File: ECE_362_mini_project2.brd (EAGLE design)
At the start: 71.1 x 35.2 mm, 18 parts

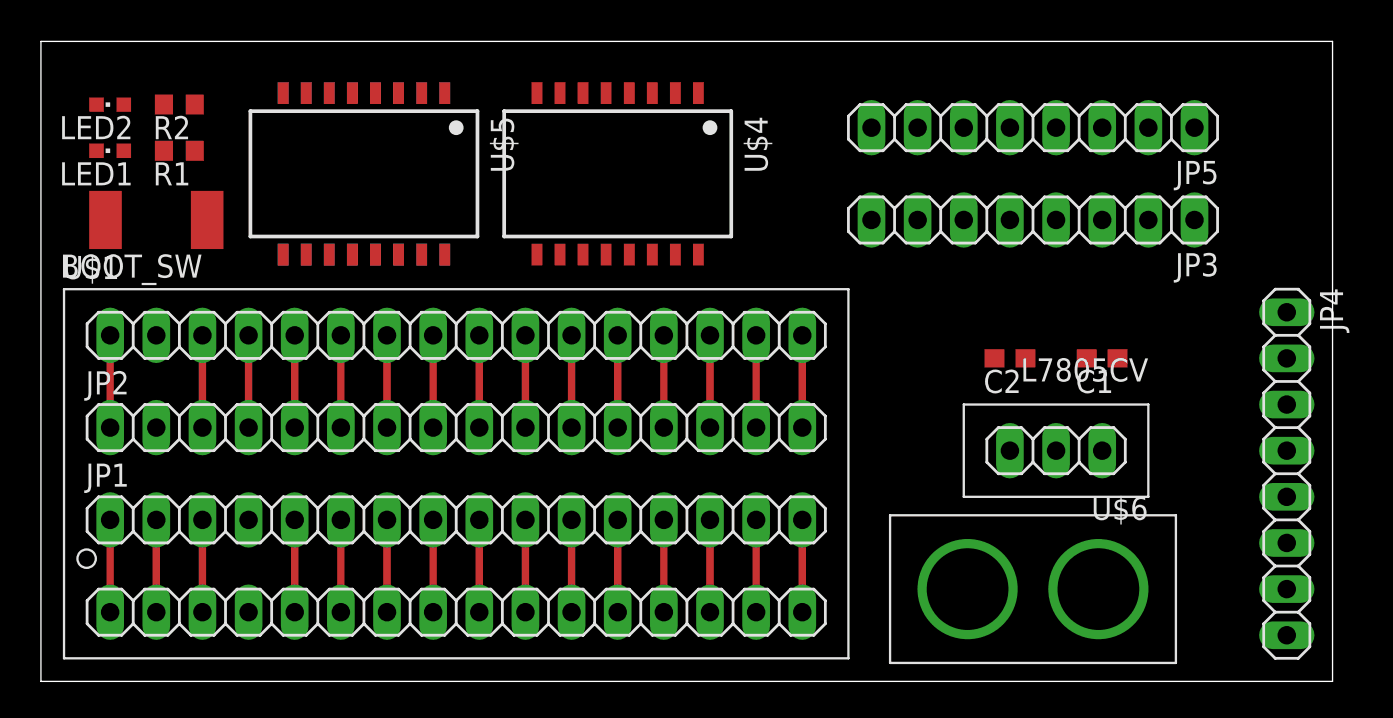
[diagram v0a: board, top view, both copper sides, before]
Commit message: Updated the board
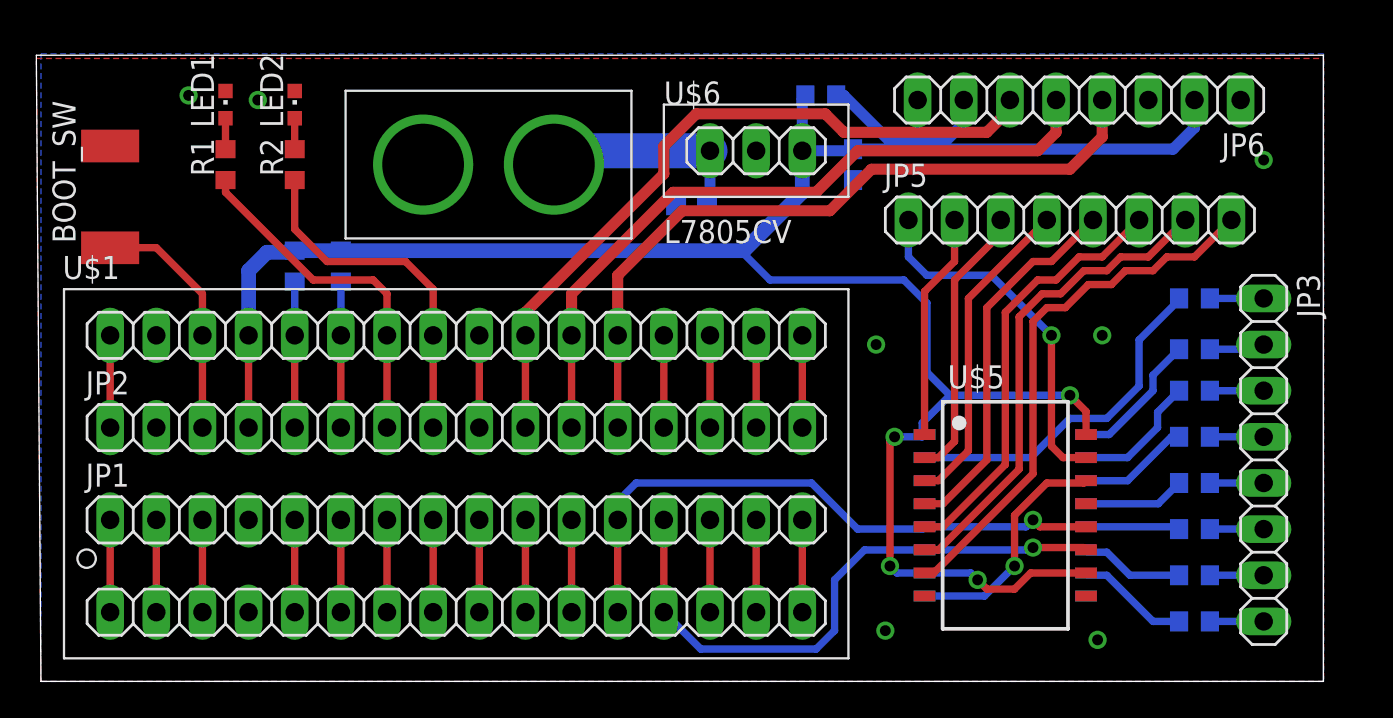
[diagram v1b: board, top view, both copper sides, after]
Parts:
- removed JP4: (no value), pinhead:1X08
- removed U$4: SHIFT_REGISTER, mini_project_parts:N5
- added JP6: (no value), pinhead:1X08
- added R10, R11, R12, R20, R5, R6, R7, R8, R9: 220, resistor:R0603
- added R3, R4: 10k, resistor:R0603
- moved U$2 40.0 mm to (53.1, 9.14), turned to 270 degrees
- moved U$5 40.0 mm to (53.1, 9.14), turned to 270 degrees
- moved U$3 38.0 mm to (24.6, 28.4)
- moved U$6 29.0 mm to (34.3, 26.7), turned to 0 degrees
- moved C1 24.1 mm to (35.8, 26.2), flipped to the bottom
- moved JP3 18.3 mm to (67.3, 12.2), turned to 270 degrees
- moved C2 13.7 mm to (44.7, 28.4), flipped to the bottom, turned to 270 degrees
- moved LED2 10.2 mm to (14.0, 31.8), turned to 0 degrees
- moved R2 7.16 mm to (14.0, 28.4), turned to 90 degrees
- moved LED1 6.84 mm to (10.2, 31.8), turned to 0 degrees
- moved JP5 5.47 mm to (56.6, 25.4), turned to 0 degrees
- moved BOOT_SW 2.84 mm to (3.81, 26.7), turned to 90 degrees
- moved R1 2.65 mm to (10.2, 28.4), turned to 90 degrees
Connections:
- removed net LED2_Q0: JP4.1, U$2.9, U$4.15
- removed net LED2_Q1: JP4.2, U$4.1
- removed net LED2_Q2: JP4.3, U$4.2
- removed net LED2_Q3: JP4.4, U$4.3
- removed net LED2_Q4: JP4.5, U$4.4
- removed net LED2_Q5: JP4.6, U$4.5
- removed net LED2_Q6: JP4.7, U$4.6
- removed net LED2_Q7: JP4.8, U$4.7
- new net A0: R20.1, U$2.15
- new net A1: R6.1, U$2.1
- new net A2: R7.1, U$2.2
- new net A3: R8.1, U$2.3
- new net A4: R9.1, U$2.4
- new net A5: R10.1, U$2.5
- new net A7: R12.1, U$2.7
- new net N$3: R11.1, U$2.6
- new net N$4: U$2.9, U$5.14
- new net N$5: U$2.14
- new net N$9: JP6.7, R5.2
- net +5V: now also JP6.2, R3.2, R4.2, R5.1, U$2.10, U$5.10; no longer U$4.16
- net AN7: now also U$2.12, U$5.12
- net GND: now also JP6.1, JP6.3, JP6.8, U$2.13, U$5.13; no longer U$4.8
- net LCD_Q0: no longer U$4.9
- net LED1_Q0: now also R20.2; no longer U$2.15
- net LED1_Q1: now also R6.2; no longer U$2.1
- net LED1_Q2: now also R7.2; no longer U$2.2
- net LED1_Q3: now also R8.2; no longer U$2.3
- net LED1_Q4: now also R9.2; no longer U$2.4
- net LED1_Q5: now also R10.2; no longer U$2.5
- net LED1_Q6: now also R11.2; no longer U$2.6
- net LED1_Q7: now also R12.2; no longer U$2.7
- net PE0: now also R3.1
- net PE1: now also R4.1
- net PM5: now also U$2.11, U$5.11
- net PT2: now also JP6.4
- net PT3: now also JP6.5
- net PT4: now also JP6.6
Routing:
- net +5V: track 5.08 -> 119.7 mm, vias 0 -> 4
- net PT2: track 5.08 -> 40.2 mm
- net PT4: track 5.08 -> 39.9 mm
- net PT3: track 5.08 -> 39.5 mm
- net LCD_Q7: track 0.00 -> 29.8 mm
- net AN7: track 5.08 -> 33.7 mm, vias 0 -> 1
- net PM5: track 5.08 -> 33.1 mm, vias 0 -> 1
- net LCD_Q6: track 0.00 -> 26.8 mm
- net LCD_Q5: track 0.00 -> 23.7 mm
- net LCD_Q4: track 0.00 -> 20.7 mm
- net LCD_Q0: track 0.00 -> 20.0 mm, vias 0 -> 1
- net A0: track 0.00 -> 19.2 mm
- net LCD_Q3: track 0.00 -> 17.6 mm
- net LCD_Q2: track 0.00 -> 15.3 mm
- net PT6: track 5.08 -> 19.3 mm
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- added copper zone on layer 1, net GND
- added copper zone on layer 16, net GND
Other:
- board size 71.1 x 35.2 mm -> 70.8 x 34.5 mm
